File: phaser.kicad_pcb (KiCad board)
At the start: 2 copper layers, 58 x 78 mm, 127 parts, among them J1 Res, J10 Frq, J11 Wvf, J12 Boot, J13 Stage, J14 Tap, J15 CV, J2 PWR, J3 In, J4 Out, J5 Dep, J6 ISP, J7 Dep, J8 USB, J9 Exp, Q1 BC846, U1 L7805, U2 TL074, U3 TL074, U4 TL074, U5 TL074, U6 ATmega32U2-AU, Y1 16 MHz

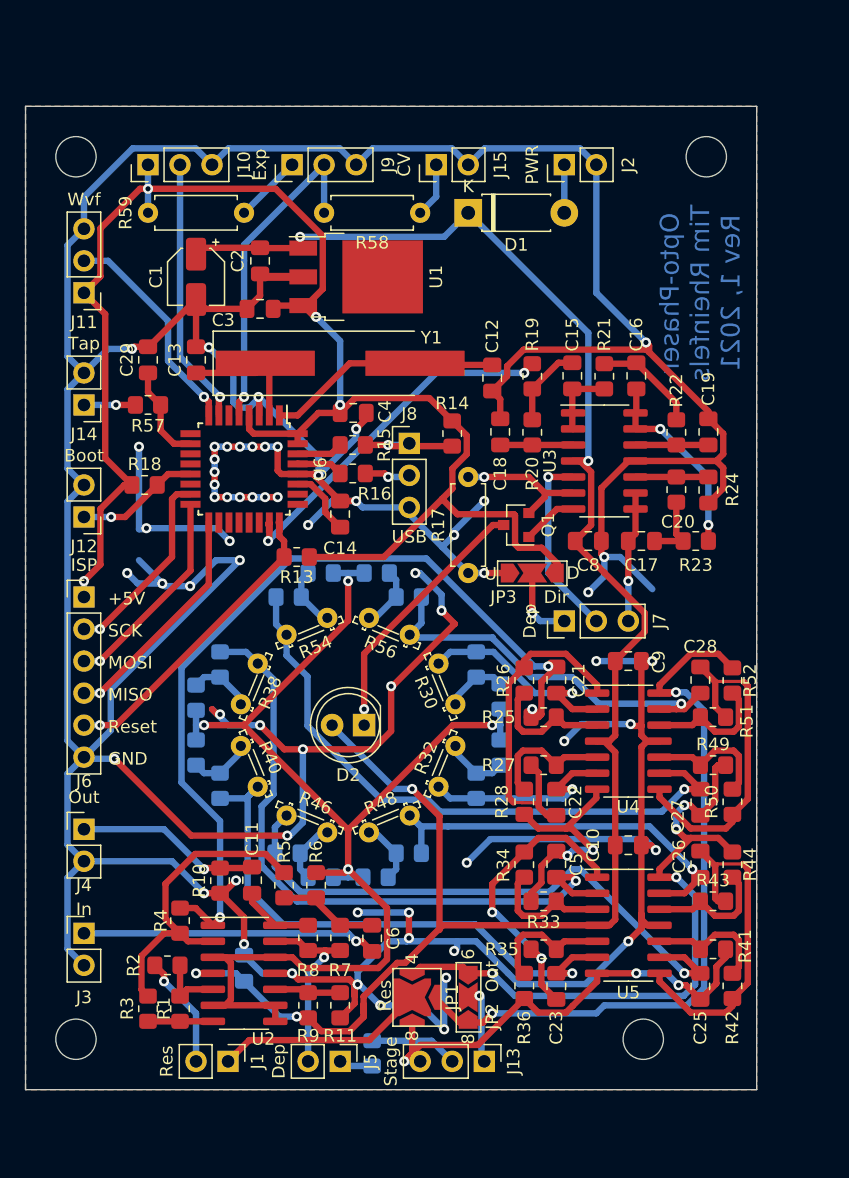
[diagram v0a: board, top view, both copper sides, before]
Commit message: Revision 2
See changelog.txt
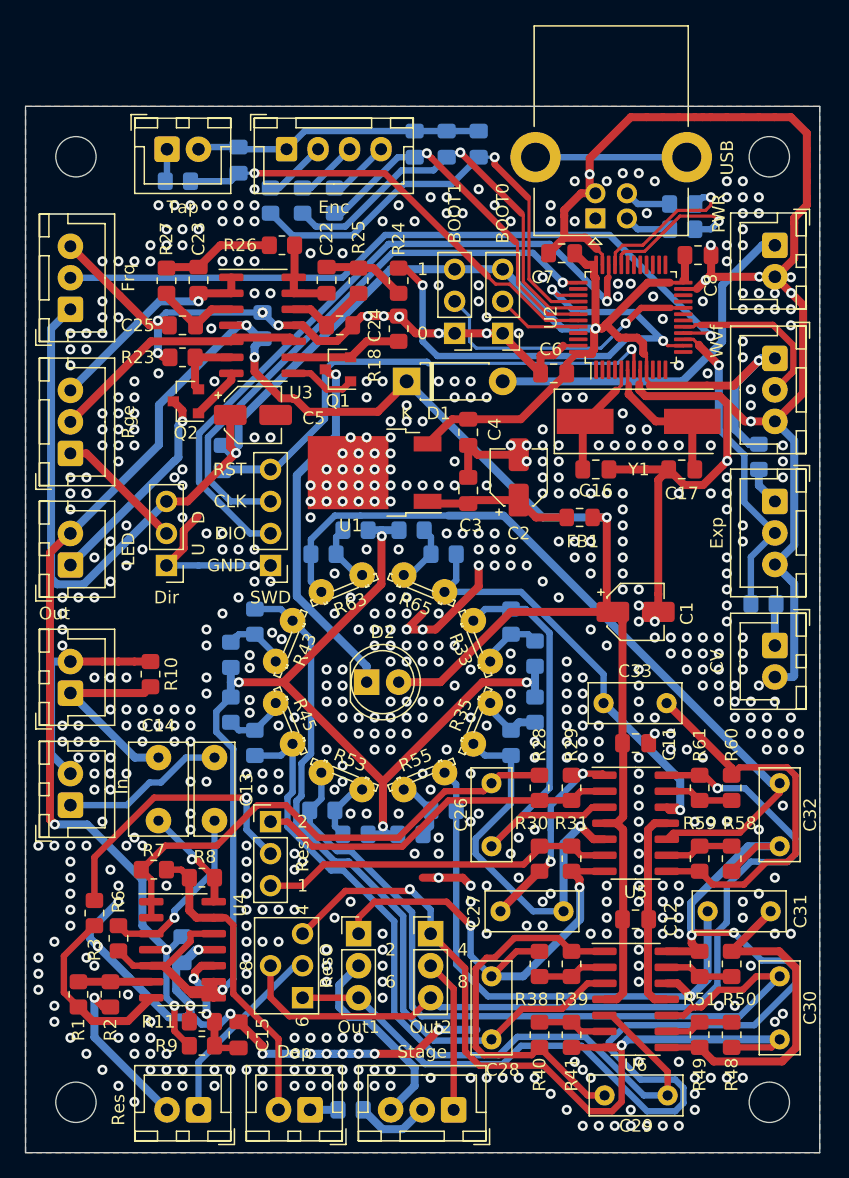
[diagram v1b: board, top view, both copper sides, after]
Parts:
- removed the C12 at (146.7, 67.7)
- removed the C13 at (123.2, 66.3)
- removed the C14 at (134.6, 78.5)
- removed the C22 at (151.8, 101.4)
- removed the C23 at (151.8, 116.0)
- removed the C25 at (163.2, 116.0)
- removed the J13 at (146.1, 121.9)
- removed the J8 at (140.1, 72.9)
- removed the J9 at (130.8, 50.8)
- removed JP2: Out, Jumper:SolderJumper-3_P2.0mm_Open_TrianglePad1.0x1.5mm_NumberLabels
- removed JP3: Dir, Jumper:SolderJumper-3_P2.0mm_Open_TrianglePad1.0x1.5mm_NumberLabels
- removed the R14 at (143.5, 72.1)
- removed the R16 at (135.6, 75.3)
- removed the R18 at (119.1, 76.2)
- removed the R24 at (161.3, 76.6)
- removed R4, R5: 10k, Resistor_SMD:R_0805_2012Metric_Pad1.20x1.40mm_HandSolder
- removed the U6 at (127.0, 74.9)
- added C10: 100n, Capacitor_SMD:C_0805_2012Metric_Pad1.18x1.45mm_HandSolder, B.Cu at (122.1, 113.1)
- added C15: 22n, Capacitor_SMD:C_0805_2012Metric_Pad1.18x1.45mm_HandSolder, F.Cu at (126.6, 119.8)
- added C16: 15p, Capacitor_SMD:C_0805_2012Metric_Pad1.18x1.45mm_HandSolder, F.Cu at (154.9, 75.0)
- added C19: 100n, Capacitor_SMD:C_0805_2012Metric_Pad1.18x1.45mm_HandSolder, B.Cu at (145.6, 49.2)
- added C2: 10u, Capacitor_SMD:CP_Elec_4x5.4, F.Cu at (148.8, 75.6)
- added C29: 22n, Capacitor_THT:C_Rect_L7.2mm_W3.0mm_P5.00mm_FKS2_FKP2_MKS2_MKP2, F.Cu at (160.6, 124.6)
- added C30: 22n, Capacitor_THT:C_Rect_L7.2mm_W3.0mm_P5.00mm_FKS2_FKP2_MKS2_MKP2, F.Cu at (169.5, 115.2)
- added C31: 22n, Capacitor_THT:C_Rect_L7.2mm_W3.0mm_P5.00mm_FKS2_FKP2_MKS2_MKP2, F.Cu at (163.8, 110.0)
- added C32: 22n, Capacitor_THT:C_Rect_L7.2mm_W3.0mm_P5.00mm_FKS2_FKP2_MKS2_MKP2, F.Cu at (169.5, 99.9)
- added C33: 22n, Capacitor_THT:C_Rect_L7.2mm_W3.0mm_P5.00mm_FKS2_FKP2_MKS2_MKP2, F.Cu at (155.5, 93.5)
- added C7: 100n, Capacitor_SMD:C_0805_2012Metric_Pad1.18x1.45mm_HandSolder, F.Cu at (152.2, 57.8)
- added FB1: Ferrite_Bead, Inductor_SMD:L_0805_2012Metric_Pad1.15x1.40mm_HandSolder, F.Cu at (153.6, 78.8)
- added J15: Frq, Connector_JST:JST_XH_B3B-XH-A_1x03_P2.50mm_Vertical, F.Cu at (113.2, 62.3)
- added J16: Wvf, Connector_JST:JST_XH_B3B-XH-A_1x03_P2.50mm_Vertical, F.Cu at (169.1, 66.2)
- added J17: Tap, Connector_JST:JST_XH_B2B-XH-A_1x02_P2.50mm_Vertical, F.Cu at (120.9, 49.6)
- added J18: BOOT0, Connector_PinHeader_2.54mm:PinHeader_1x03_P2.54mm_Vertical, F.Cu at (147.5, 64.2)
- added J19: LED, Connector_JST:JST_XH_B2B-XH-A_1x02_P2.50mm_Vertical, F.Cu at (113.2, 82.5)
- added J20: BOOT1, Connector_PinHeader_2.54mm:PinHeader_1x03_P2.54mm_Vertical, F.Cu at (143.7, 64.2)
- added J21: Enc, Connector_JST:JST_XH_B4B-XH-A_1x04_P2.50mm_Vertical, F.Cu at (130.4, 49.6)
- added J22: ResI, Connector_PinHeader_2.54mm:PinHeader_1x03_P2.54mm_Vertical, F.Cu at (129.1, 102.9)
- added J5: Out1, Connector_PinHeader_2.54mm:PinHeader_1x03_P2.54mm_Vertical, F.Cu at (136.1, 111.8)
- added J7: Stage, Connector_JST:JST_XH_B3B-XH-A_1x03_P2.50mm_Vertical, F.Cu at (143.6, 125.8)
- added Q2: BC846, Package_TO_SOT_SMD:SOT-23, F.Cu at (122.4, 69.6)
- added R17: 22, Resistor_SMD:R_0805_2012Metric_Pad1.20x1.40mm_HandSolder, B.Cu at (161.8, 55.9)
- added R20: 10k, Resistor_SMD:R_0805_2012Metric_Pad1.20x1.40mm_HandSolder, B.Cu at (134.2, 53.6)
- added R21: 10k, Resistor_SMD:R_0805_2012Metric_Pad1.20x1.40mm_HandSolder, B.Cu at (131.6, 53.6)
- added R22: 10k, Resistor_SMD:R_0805_2012Metric_Pad1.20x1.40mm_HandSolder, B.Cu at (129.1, 53.6)
- added U4: TL074, Package_SO:SOIC-14_3.9x8.7mm_P1.27mm, F.Cu at (122.1, 113.1)
- C13: renamed from C6; footprint Capacitor_SMD:C_0805_2012Metric_Pad1.18x1.45mm_HandSolder -> Capacitor_THT:C_Rect_L7.2mm_W3.0mm_P5.00mm_FKS2_FKP2_MKS2_MKP2
- C14: renamed from C11; value 47n -> 68n; footprint Capacitor_SMD:C_0805_2012Metric_Pad1.18x1.45mm_HandSolder -> Capacitor_THT:C_Rect_L7.2mm_W4.5mm_P5.00mm_FKS2_FKP2_MKS2_MKP2
- C17: value 15n -> 15p
- C18: renamed from C29; moved to B.Cu
- C20: value 15n -> 100n; moved to B.Cu
- C21: value C_Small -> 100n; moved to B.Cu
- C26, C27, C28: value C_Small -> 22n; footprint Capacitor_SMD:C_0805_2012Metric_Pad1.18x1.45mm_HandSolder -> Capacitor_THT:C_Rect_L7.2mm_W3.0mm_P5.00mm_FKS2_FKP2_MKS2_MKP2
- C5: value C_Small -> 10u; footprint Capacitor_SMD:C_0805_2012Metric_Pad1.18x1.45mm_HandSolder -> Capacitor_SMD:CP_Elec_4x5.4
- H1, H2, H3, H4: value MountingHole -> (none)
- J1, J2, J3, J4: footprint Connector_PinHeader_2.54mm:PinHeader_1x02_P2.54mm_Vertical -> Connector_JST:JST_XH_B2B-XH-A_1x02_P2.50mm_Vertical
- J10: value Frq -> SWD; footprint Connector_PinHeader_2.54mm:PinHeader_1x03_P2.54mm_Vertical -> Connector_PinHeader_2.54mm:PinHeader_1x04_P2.54mm_Vertical
- J11: value Wvf -> Dir
- J12: value Boot -> Exp; footprint Connector_PinHeader_2.54mm:PinHeader_1x02_P2.54mm_Vertical -> Connector_JST:JST_XH_B3B-XH-A_1x03_P2.50mm_Vertical
- J13: renamed from J7; value Dep -> Rge; footprint Connector_PinHeader_2.54mm:PinHeader_1x03_P2.54mm_Vertical -> Connector_JST:JST_XH_B3B-XH-A_1x03_P2.50mm_Vertical
- J14: value Tap -> USB; footprint Connector_PinHeader_2.54mm:PinHeader_1x02_P2.54mm_Vertical -> Connector_USB:USB_B_Lumberg_2411_02_Horizontal
- J6: value ISP -> Out2; footprint Connector_PinHeader_2.54mm:PinHeader_1x06_P2.54mm_Vertical -> Connector_PinHeader_2.54mm:PinHeader_1x03_P2.54mm_Vertical
- J8: renamed from J5; footprint Connector_PinHeader_2.54mm:PinHeader_1x02_P2.54mm_Vertical -> Connector_JST:JST_XH_B2B-XH-A_1x02_P2.50mm_Vertical
- J9: renamed from J15; footprint Connector_PinHeader_2.54mm:PinHeader_1x02_P2.54mm_Vertical -> Connector_JST:JST_XH_B2B-XH-A_1x02_P2.50mm_Vertical
- JP1: value Res -> ResO; footprint phaser:SolderJumper4_Open -> phaser:Sel3
- R1: value 100k -> 1k
- R13: moved to B.Cu
- R14: renamed from R58; footprint Resistor_THT:R_Axial_DIN0207_L6.3mm_D2.5mm_P7.62mm_Horizontal -> Resistor_SMD:R_0805_2012Metric_Pad1.20x1.40mm_HandSolder; moved to B.Cu
- R15: renamed from R59; footprint Resistor_THT:R_Axial_DIN0207_L6.3mm_D2.5mm_P7.62mm_Horizontal -> Resistor_SMD:R_0805_2012Metric_Pad1.20x1.40mm_HandSolder; moved to B.Cu
- R16: renamed from R15; moved to B.Cu
- R18: renamed from R17; value 250 -> 165; footprint Resistor_THT:R_Axial_DIN0207_L6.3mm_D2.5mm_P7.62mm_Horizontal -> Resistor_SMD:R_0805_2012Metric_Pad1.20x1.40mm_HandSolder
- R19: renamed from R57; moved to B.Cu
- R2: value 1k -> 2k
- R23: value 100k -> 165
- R32: renamed from R29; value R_Small -> 100k
- R33: renamed from R30; value R_PHOTO -> 2k-230k
- R34: renamed from R31; value R_Small -> 100k
- R35: renamed from R32; value R_PHOTO -> 2k-230k
- R36: renamed from R60; value R_Small -> 10k
- R37: renamed from R61; value R_Small -> 10k
- R42: renamed from R37; value R_Small -> 100k
- R43: renamed from R38; value R_PHOTO -> 2k-230k
- R44: renamed from R39; value R_Small -> 100k
- R45: renamed from R40; value R_PHOTO -> 2k-230k
- R46: renamed from R62; value R_Small -> 10k
- R47: renamed from R63; value R_Small -> 10k
- R52: renamed from R45; value R_Small -> 100k
- R53: renamed from R46; value R_PHOTO -> 2k-230k
- R54: renamed from R47; value R_Small -> 100k
- R55: renamed from R48; value R_PHOTO -> 2k-230k
- R56: renamed from R64; value R_Small -> 10k
- R57: renamed from R65; value R_Small -> 10k
- R62: renamed from R53; value R_Small -> 100k
- R63: renamed from R54; value R_PHOTO -> 2k-230k
- R64: renamed from R55; value R_Small -> 100k
- R65: renamed from R56; value R_PHOTO -> 2k-230k
- R66, R67: value R_Small -> 10k
- U1: value L7805 -> LF33; footprint Package_TO_SOT_SMD:TO-252-3_TabPin4 -> Package_TO_SOT_SMD:TO-252-2
- U2: value TL074 -> STM32L151CBTxA; footprint Package_SO:SOIC-14_3.9x8.7mm_P1.27mm -> Package_QFP:LQFP-48_7x7mm_P0.5mm
- U3: value TL074 -> LM324
- Y1: footprint Crystal:Crystal_SMD_HC49-SD_HandSoldering -> Crystal:Crystal_SMD_HC49-SD
- moved U2 60.4 mm to (157.7, 62.9), turned to 90 degrees
- moved J12 54.8 mm to (169.1, 77.5), turned to 270 degrees
- moved R15 52.2 mm to (167.8, 74.0), turned to 270 degrees
- moved C9 51.0 mm to (128.5, 63.6)
- moved J9 46.6 mm to (169.1, 88.9), turned to 270 degrees
- moved C21 44.0 mm to (140.5, 49.2)
- moved C1 43.8 mm to (158.1, 86.3), turned to 0 degrees
- moved R23 43.2 mm to (122.1, 66.1)
- moved J14 43.2 mm to (154.9, 55.1), turned to 90 degrees
- moved C5 43.0 mm to (127.7, 70.6), turned to 0 degrees
- moved C25 42.6 mm to (122.1, 63.5), turned to 0 degrees
- moved R27 42.2 mm to (120.8, 60.0)
- moved J13 41.4 mm to (113.2, 73.7)
- moved R14 41.3 mm to (168.2, 85.6)
- moved J6 38.3 mm to (141.8, 111.8)
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- renumbered C9 to C11, C10 to C12, C15 to C22, C16 to C23, C18 to C24, C19 to C25, C2 to C3, C3 to C4, C4 to C6, C7 to C9, R19 to R24, R20 to R25, R21 to R26, R22 to R27, R25 to R28, R26 to R29, R27 to R30, R28 to R31, R33 to R38, R34 to R39, R35 to R40, R36 to R41, R41 to R48, R42 to R49, R43 to R50, R44 to R51, R49 to R58, R50 to R59, R51 to R60, R52 to R61, U4 to U5, U5 to U6
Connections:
- C13 pad 1: Net-(C6-Pad1) -> Net-(C13-Pad1)
- C14 pad 2: Net-(C11-Pad2) -> Net-(C14-Pad2)
- C17 pad 1: /low_pass/y -> GND
- C18 pad 1: Net-(C29-Pad1) -> Tap
- C20 pad 1: GND -> ENC_B
- C20 pad 2: Net-(C20-Pad2) -> GND
- C21 pad 1: Net-(C21-Pad1) -> ENC_S
- C21 pad 2: /stage_12/u -> GND
- C22 pad 1: Net-(C15-Pad1) -> Net-(C22-Pad1)
- C23 pad 1: Net-(C16-Pad1) -> /low_pass/y
- C24 pad 2: Net-(C18-Pad2) -> Net-(C24-Pad2)
- C25 pad 2: Net-(C19-Pad2) -> Net-(C25-Pad2)
- C26 pad 2: Net-(C26-Pad2) -> /stage_12/u
- C27 pad 2: /stage_78/u -> Net-(C27-Pad2)
- C28 pad 2: Net-(C28-Pad2) -> /stage_34/u
- C3 pad 1: +9V -> Net-(C2-Pad1)
- C4 pad 1: +5V -> +3V3
- C5 pad 1: Net-(C5-Pad1) -> +3V3
- C5 pad 2: /stage_34/u -> GND
- C6 pad 2: +5V -> +3V3
- C8 pad 1: +9V -> GND
- C8 pad 2: GND -> +3V3
- J10 pad 1: +5V -> GND
- J10 pad 2: Net-(J10-Pad2) -> SWDIO
- J10 pad 3: GND -> SWCLK
- J11 pad 1: +5V -> GND
- J11 pad 3: GND -> +3V3
- J12 pad 1: ~HWB -> Net-(J12-Pad1)
- J12 pad 2: GND -> CV
- J13 pad 1: Net-(J7-Pad1) -> Net-(J11-Pad2)
- J13 pad 2: Net-(J7-Pad2) (its old number) -> Net-(J13-Pad2)
- J14 pad 2: GND -> Net-(J14-Pad2)
- J6 pad 1: +5V -> /stage_56/u
- J6 pad 2: SCK -> Net-(J6-Pad2)
- J6 pad 3: MOSI -> /stage_78/y
- J8 pad 2: Net-(J5-Pad2) -> Net-(J8-Pad2)
- R11 pad 1: Net-(R11-Pad1) -> Net-(C15-Pad1)
- R13 pad 1: ~RESET -> NRST
- R13 pad 2: +5V -> +3V3
- R14 pad 2: Net-(J9-Pad2) -> CV
- R15 pad 1: +5V -> +3V3
- R15 pad 2: Net-(J9-Pad1) (its old number) -> Net-(J12-Pad1)
- R16 pad 1: Net-(J8-Pad1) (its old number) -> Net-(J14-Pad3)
- R16 pad 2: D- -> D+
- R19 pad 1: Net-(C29-Pad1) -> Tap
- R19 pad 2: Net-(J14-Pad1) -> Net-(J17-Pad1)
- R23 pad 1: Net-(C17-Pad2) -> GND
- R23 pad 2: Net-(C16-Pad1) -> Net-(Q2-Pad2)
- R24 pad 2: PWM -> DAC
- R25 pad 1: Net-(C18-Pad2) -> Net-(C24-Pad2)
- R26 pad 2: Net-(C15-Pad1) -> Net-(C22-Pad1)
- R27 pad 1: Net-(C19-Pad2) -> Net-(C25-Pad2)
- R28 pad 1: Net-(R25-Pad1) -> /stage_12/res1
- R29 pad 1: Net-(C22-Pad2) (its old number) -> Net-(C27-Pad2)
- R29 pad 2: Net-(R25-Pad1) -> /stage_12/res1
- R3 pad 1: Net-(R3-Pad1) -> Net-(R1-Pad2)
- R3 pad 2: Net-(R1-Pad2) -> Net-(J22-Pad2)
- R30 pad 1: Net-(R27-Pad1) -> /stage_12/res2
- R30 pad 2: Net-(C22-Pad2) (its old number) -> Net-(C27-Pad2)
- R31 pad 2: Net-(R27-Pad1) -> /stage_12/res2
- R32 pad 1: Net-(C21-Pad1) -> Net-(C26-Pad1)
- R33 pad 2: Net-(C21-Pad1) -> Net-(C26-Pad1)
- R34 pad 1: Net-(C22-Pad1) -> Net-(C27-Pad1)
- R35 pad 1: Net-(C22-Pad1) -> Net-(C27-Pad1)
- R38 pad 1: Net-(R33-Pad1) -> Net-(R38-Pad1)
- R39 pad 2: Net-(R33-Pad1) -> Net-(R38-Pad1)
- R40 pad 1: Net-(R35-Pad1) -> Net-(R40-Pad1)
- R41 pad 2: Net-(R35-Pad1) -> Net-(R40-Pad1)
- R42 pad 1: Net-(C5-Pad1) -> Net-(C28-Pad1)
- R43 pad 1: Net-(C5-Pad1) -> Net-(C28-Pad1)
- R44 pad 1: Net-(C23-Pad1) -> Net-(C29-Pad1)
- R45 pad 2: Net-(C23-Pad1) -> Net-(C29-Pad1)
- R48 pad 1: Net-(R41-Pad1) -> Net-(R48-Pad1)
- R49 pad 1: Net-(C26-Pad2) -> Net-(C31-Pad2)
- R49 pad 2: Net-(R41-Pad1) -> Net-(R48-Pad1)
- R50 pad 1: Net-(R43-Pad1) -> Net-(R50-Pad1)
- R50 pad 2: Net-(C26-Pad2) -> Net-(C31-Pad2)
- R51 pad 2: Net-(R43-Pad1) -> Net-(R50-Pad1)
- R52 pad 1: Net-(C25-Pad1) -> Net-(C30-Pad1)
- R53 pad 1: Net-(C25-Pad1) -> Net-(C30-Pad1)
- R54 pad 1: Net-(C26-Pad1) -> Net-(C31-Pad1)
- R55 pad 2: Net-(C26-Pad1) -> Net-(C31-Pad1)
- R58 pad 1: Net-(R49-Pad1) -> Net-(R58-Pad1)
- R59 pad 1: Net-(C28-Pad2) -> Net-(C33-Pad2)
- R59 pad 2: Net-(R49-Pad1) -> Net-(R58-Pad1)
- R6 pad 2: Net-(C6-Pad1) -> Net-(C13-Pad1)
- R60 pad 1: Net-(R51-Pad1) -> Net-(R60-Pad1)
- R60 pad 2: Net-(C28-Pad2) -> Net-(C33-Pad2)
- R61 pad 2: Net-(R51-Pad1) -> Net-(R60-Pad1)
- R62 pad 1: Net-(C27-Pad1) -> Net-(C32-Pad1)
- R63 pad 2: Net-(C27-Pad1) -> Net-(C32-Pad1)
- R64 pad 1: Net-(C28-Pad1) -> Net-(C33-Pad1)
- R65 pad 1: Net-(C28-Pad1) -> Net-(C33-Pad1)
- R7 pad 1: Net-(J5-Pad2) -> Net-(J8-Pad2)
- R7 pad 2: Net-(C6-Pad1) -> /stage_12/u
- R8 pad 1: Net-(C11-Pad2) -> Net-(C14-Pad2)
- R8 pad 2: Net-(J5-Pad2) -> Net-(J8-Pad2)
- R9 pad 2: Net-(R11-Pad1) -> Net-(C15-Pad1)
- U1 pad 1: +9V -> Net-(C2-Pad1)
- U1 pad 3: +5V -> +3V3
- U2 pad 1: /stage_12/u -> Net-(U2-Pad1)
- U2 pad 10: Net-(R11-Pad1) -> Net-(U2-Pad10)
- U2 pad 11: GND -> Net-(U2-Pad11)
- U2 pad 12: GNDA -> Net-(U2-Pad12)
- U2 pad 13: Net-(J5-Pad2) -> Net-(U2-Pad13)
- U2 pad 14: Net-(C11-Pad2) -> DAC
- U2 pad 2: Net-(R3-Pad1) -> Net-(U2-Pad2)
- U2 pad 3: GNDA -> Net-(U2-Pad3)
- U2 pad 4: +9V -> Net-(U2-Pad4)
- U2 pad 5: Net-(R1-Pad1) -> Net-(C16-Pad2)
- U2 pad 6: GNDA -> Net-(C17-Pad2)
- U2 pad 7: Net-(R1-Pad2) -> NRST
- U2 pad 8: GNDA -> GND
- U2 pad 9: GNDA -> +3V3
- U3 pad 1: Net-(C15-Pad1) -> /low_pass/y
- U3 pad 10: Net-(C20-Pad2) -> Net-(J13-Pad2)
- U3 pad 12: Net-(C19-Pad2) -> Net-(C24-Pad2)
- U3 pad 13: Net-(C16-Pad1) -> Net-(C22-Pad1)
- U3 pad 14: Net-(C16-Pad1) -> Net-(C22-Pad1)
- U3 pad 2: Net-(C15-Pad1) -> /low_pass/y
- U3 pad 3: Net-(C18-Pad2) -> Net-(C25-Pad2)
- U3 pad 5: Net-(J7-Pad2) (its old number) -> Net-(J13-Pad2)
- U3 pad 6: Net-(Q1-Pad2) -> Net-(Q2-Pad2)
- U3 pad 7: Net-(Q1-Pad1) -> Net-(Q2-Pad1)
- U3 pad 8: /low_pass/y -> Net-(Q1-Pad1)
- U3 pad 9: /low_pass/y -> Net-(Q1-Pad2)
- U5 pad 1: Net-(C22-Pad2) (its old number) -> Net-(C27-Pad2)
- U5 pad 10: Net-(R49-Pad1) -> Net-(C32-Pad1)
- U5 pad 12: Net-(R51-Pad1) -> Net-(C33-Pad1)
- U5 pad 13: Net-(C28-Pad1) -> Net-(R60-Pad1)
- U5 pad 2: Net-(C21-Pad1) -> /stage_12/res1
- U5 pad 3: Net-(R25-Pad1) -> Net-(C26-Pad1)
- U5 pad 5: Net-(R27-Pad1) -> Net-(C27-Pad1)
- U5 pad 6: Net-(C22-Pad1) -> /stage_12/res2
- U5 pad 8: Net-(C28-Pad2) -> Net-(C33-Pad2)
- U5 pad 9: Net-(C27-Pad1) -> Net-(R58-Pad1)
- U6 pad 10: Net-(R41-Pad1) -> Net-(C30-Pad1)
- U6 pad 12: Net-(R43-Pad1) -> Net-(C31-Pad1)
- U6 pad 13: Net-(C26-Pad1) -> Net-(R50-Pad1)
- U6 pad 2: Net-(C5-Pad1) -> Net-(R38-Pad1)
- U6 pad 3: Net-(R33-Pad1) -> Net-(C28-Pad1)
- U6 pad 5: Net-(R35-Pad1) -> Net-(C29-Pad1)
- U6 pad 6: Net-(C23-Pad1) -> Net-(R40-Pad1)
- U6 pad 8: Net-(C26-Pad2) -> Net-(C31-Pad2)
- U6 pad 9: Net-(C25-Pad1) -> Net-(R48-Pad1)
- Y1 pad 1: Net-(C13-Pad1) -> Net-(C16-Pad2)
- Y1 pad 2: Net-(C12-Pad1) -> Net-(C17-Pad2)
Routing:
- net GND: track 527.4 -> 336.0 mm, vias 62 -> 650
- net +3V3: track 0.00 -> 154.0 mm, vias 0 -> 3
- net +5V: track 129.5 -> 0.00 mm, vias 4 -> 0
- net Net-(C30-Pad1): track 0.00 -> 64.0 mm
- net Net-(C32-Pad1): track 0.00 -> 62.6 mm
- net Frq: track 0.00 -> 58.0 mm, vias 0 -> 1
- net SWDIO: track 0.00 -> 57.2 mm, vias 0 -> 1
- net Net-(C29-Pad1): track 7.78 -> 63.4 mm
- net Net-(C5-Pad1): track 53.0 -> 0.00 mm, vias 1 -> 0
- net Net-(C25-Pad1): track 49.8 -> 0.00 mm, vias 1 -> 0
- net SWCLK: track 0.00 -> 45.6 mm, vias 0 -> 1
- net Net-(C23-Pad1): track 45.4 -> 0.00 mm, vias 1 -> 0
- net Net-(C31-Pad1): track 0.00 -> 44.9 mm, vias 0 -> 1
- net DAC: track 0.00 -> 41.7 mm, vias 0 -> 3
- net NRST: track 0.00 -> 40.5 mm, vias 0 -> 1
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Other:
- board size 58 x 78 mm -> 63 x 83 mm
- rule trace_min: 0.2 -> 0.254
- rule via_min_size: 0.4 -> 0.254
- board text added: "0"
- board text added: "1"
- board text added: "2"
- board text added: "4"
- board text added: "6"
- board text added: "8"
- board text added: "CLK"
- board text added: "D"
- board text added: "DIO"
- board text added: "Optophaser Rev 2, 2021 Tim Rheinfels"
- board text added: "RST"
- board text added: "U"
- board text removed: "+5V"
- board text removed: "MISO"
- board text removed: "MOSI"
- board text removed: "Opto-Phaser Tim Rheinfels Rev 1, 2021"
- board text removed: "Reset"
- board text removed: "SCK"
